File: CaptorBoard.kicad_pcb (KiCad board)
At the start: 2 copper layers, 90 x 50 mm, 56 parts, among them J2 Screw_Terminal_01x03, J3 Screw_Terminal_01x03, J5 Conn_01x04, J7 Conn_01x08, K1 G5LE-1-DC5, K2 G5LE-1-DC5, Q1 2N7002E, Q2 2N7002E, SW1 SW_PUSH, SW2 SW_PUSH, U1 ESP32-WROOM-32E-N4, U2 TC1264-3.3VDBTR, U3 MOC3041M-opto, U4 MOC3041M-opto, Y1 CM8V-T1A-32.768kHz-12.5pF-20P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

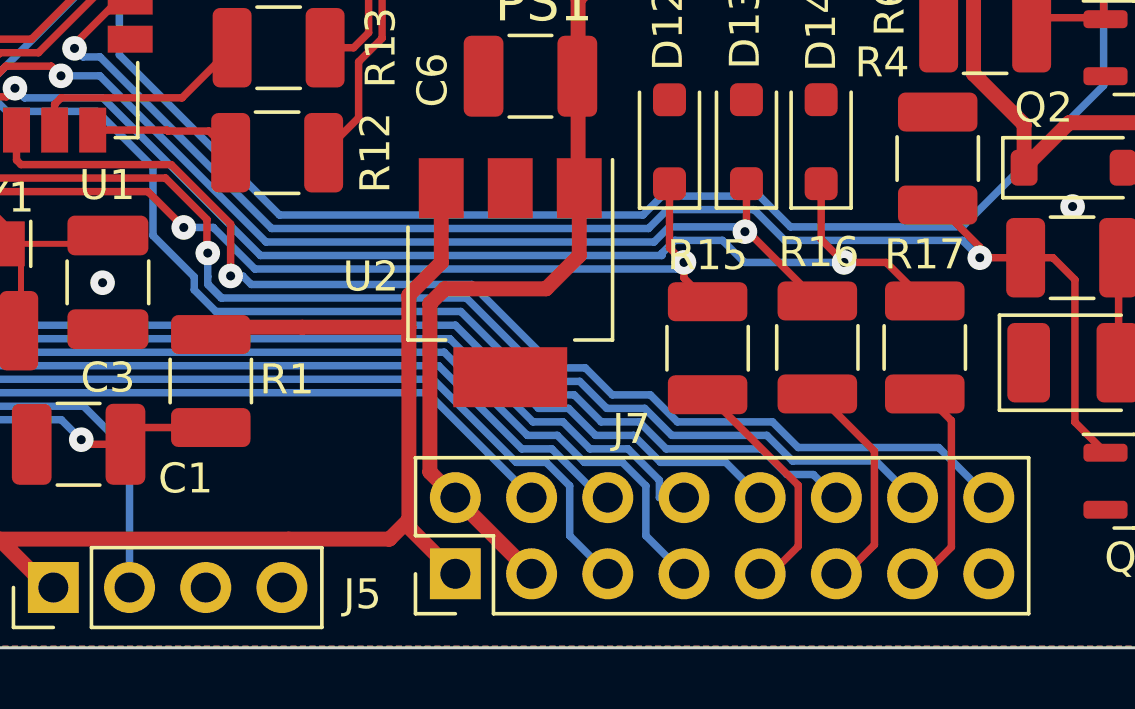
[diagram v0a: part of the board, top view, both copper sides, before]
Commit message: change route
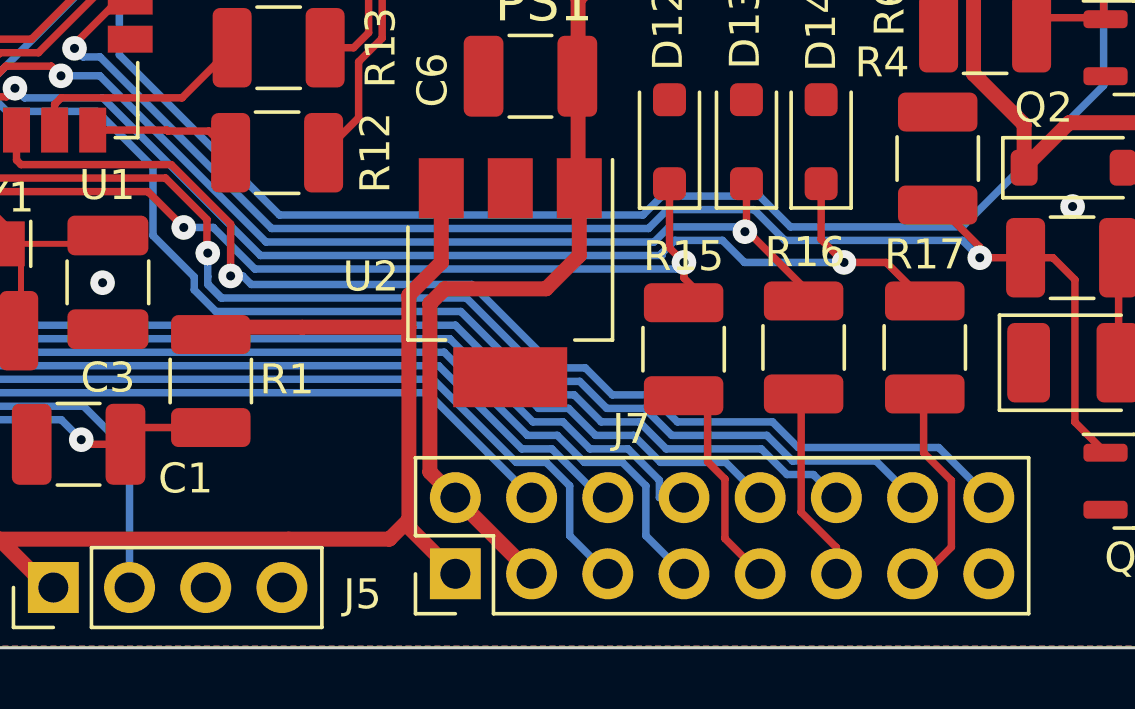
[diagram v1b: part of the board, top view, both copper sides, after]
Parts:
- moved R15 0.80 mm to (132.5, 90.0)
- moved R16 0.46 mm to (136.5, 90.0)
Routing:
- net Net-(J7-Pin_9): track 7.95 -> 6.69 mm
- net Net-(J7-Pin_11): track 7.49 -> 6.70 mm
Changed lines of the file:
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@@
   )
   (footprint "Resistor_SMD:R_1210_3225Metric_Pad1.30x2.65mm_HandSolder" (layer "F.Cu")
-    (at 133.2992 90.017 -90)
+    (at 132.5 90.05 -90)
     (descr "Resistor SMD 1210 (3225 Metric), square (rectangular) end terminal, IPC_7351 nominal with elongated pad for handsoldering. (Body size source: IPC-SM-782 page 72, https://www.pcb-3d.com/wordpress/wp-content/uploads/ipc-sm-782a_amendment_1_and_2.pdf), generated with kicad-footprint-generator")
     (tags "resistor handsolder")
@@
   )
   (footprint "Resistor_SMD:R_1210_3225Metric_Pad1.30x2.65mm_HandSolder" (layer "F.Cu")
-    (at 136.9568 89.9916 -90)
+    (at 136.5 89.9916 -90)
     (descr "Resistor SMD 1210 (3225 Metric), square (rectangular) end terminal, IPC_7351 nominal with elongated pad for handsoldering. (Body size source: IPC-SM-782 page 72, https://www.pcb-3d.com/wordpress/wp-content/uploads/ipc-sm-782a_amendment_1_and_2.pdf), generated with kicad-footprint-generator")
     (tags "resistor handsolder")
@@
     (pts (xy 185 50) (xy 185 100))
     (height -3.5)
-    (gr_text "50,0000 mm" (at 187.35 75 90) (layer "B.Fab")
+    (gr_text "50.0000 mm" (at 187.35 75 90) (layer "B.Fab")
       (effects (font (size 1 1) (thickness 0.15)))
     )
@@
     (pts (xy 95 50) (xy 185 50))
     (height -4.5)
-    (gr_text "90,0000 mm" (at 140 44.35) (layer "B.Fab")
+    (gr_text "90.0000 mm" (at 140 44.35) (layer "B.Fab")
       (effects (font (size 1 1) (thickness 0.15)))
     )
@@
   (segment (start 131.2418 94.604299) (end 131.2418 96.266) (width 0.25) (layer "B.Cu") (net 22))
   (segment (start 106.578569 90.15) (end 124.520388 90.15) (width 0.25) (layer "B.Cu") (net 22))
+  (segment (start 132.5118 87.1562) (end 132.0292 86.6736) (width 0.25) (layer "F.Cu") (net 23))
+  (segment (start 132.0292 86.6736) (end 132.0292 84.5342) (width 0.25) (layer "F.Cu") (net 23))
+  (segment (start 132.5118 87.6796) (end 133.2992 88.467) (width 0.25) (layer "F.Cu") (net 23))
   (segment (start 108.947957 84.346917) (end 108.743917 84.346917) (width 0.25) (layer "F.Cu") (net 23))
   (segment (start 108.743917 84.346917) (end 107.723 83.326) (width 0.25) (layer "F.Cu") (net 23))
   (segment (start 114.642462 84.7962) (end 109.39724 84.7962) (width 0.25) (layer "F.Cu") (net 23))
   (segment (start 115.837331 85.991069) (end 114.642462 84.7962) (width 0.25) (layer "F.Cu") (net 23))
-  (segment (start 132.5118 87.6796) (end 133.2992 88.467) (width 0.25) (layer "F.Cu") (net 23))
   (segment (start 107.723 83.326) (end 107.723 82.746) (width 0.25) (layer "F.Cu") (net 23))
-  (segment (start 132.0292 84.5342) (end 132.0292 86.6736) (width 0.25) (layer "F.Cu") (net 23))
   (segment (start 132.5118 87.1562) (end 132.5118 87.6796) (width 0.25) (layer "F.Cu") (net 23))
   (segment (start 109.39724 84.7962) (end 108.947957 84.346917) (width 0.25) (layer "F.Cu") (net 23))
-  (segment (start 132.0292 86.6736) (end 132.5118 87.1562) (width 0.25) (layer "F.Cu") (net 23))
   (via (at 115.837331 85.991069) (size 0.82) (drill 0.3) (layers "F.Cu" "B.Cu") (net 23))
   (via (at 132.5118 87.1562) (size 0.82) (drill 0.3) (layers "F.Cu" "B.Cu") (net 23))
-  (segment (start 116.822481 85.991069) (end 118.207412 87.376) (width 0.25) (layer "B.Cu") (net 23))
-  (segment (start 132.292 87.376) (end 132.5118 87.1562) (width 0.25) (layer "B.Cu") (net 23))
-  (segment (start 115.837331 85.991069) (end 116.822481 85.991069) (width 0.25) (layer "B.Cu") (net 23))
-  (segment (start 118.207412 87.376) (end 132.292 87.376) (width 0.25) (layer "B.Cu") (net 23))
+  (segment (start 132.292 87.376) (end 118.207412 87.376) (width 0.25) (layer "B.Cu") (net 23))
+  (segment (start 118.207412 87.376) (end 116.822481 85.991069) (width 0.25) (layer "B.Cu") (net 23))
+  (segment (start 132.5118 87.1562) (end 132.292 87.376) (width 0.25) (layer "B.Cu") (net 23))
+  (segment (start 116.822481 85.991069) (end 115.837331 85.991069) (width 0.25) (layer "B.Cu") (net 23))
   (segment (start 99.469161 80.9498) (end 100.133261 80.2857) (width 0.25) (layer "F.Cu") (net 24))
   (segment (start 112.4276 70.821843) (end 111.533 69.927243) (width 0.25) (layer "F.Cu") (net 24))
@@
   (segment (start 110.758 64.171) (end 110.263 64.666) (width 0.25) (layer "F.Cu") (net 35))
   (segment (start 109.906153 80.6157) (end 109.336153 81.1857) (width 0.25) (layer "F.Cu") (net 36))
-  (segment (start 134.646953 86.131753) (end 134.543447 86.131753) (width 0.25) (layer "F.Cu") (net 36))
   (segment (start 100.103 81.746) (end 100.103 82.746) (width 0.25) (layer "F.Cu") (net 36))
   (segment (start 100.6633 81.1857) (end 100.103 81.746) (width 0.25) (layer "F.Cu") (net 36))
   (segment (start 109.336153 81.1857) (end 100.6633 81.1857) (width 0.25) (layer "F.Cu") (net 36))
   (segment (start 134.5946 86.0806) (end 134.543447 86.131753) (width 0.25) (layer "F.Cu") (net 36))
-  (segment (start 136.9568 88.4416) (end 134.646953 86.131753) (width 0.25) (layer "F.Cu") (net 36))
   (segment (start 134.5946 84.5312) (end 134.5946 86.0806) (width 0.25) (layer "F.Cu") (net 36))
   (segment (start 111.746071 80.9365) (end 111.425271 80.6157) (width 0.25) (layer "F.Cu") (net 36))
+  (segment (start 134.646953 86.131753) (end 134.543447 86.131753) (width 0.25) (layer "F.Cu") (net 36))
   (segment (start 111.425271 80.6157) (end 109.906153 80.6157) (width 0.25) (layer "F.Cu") (net 36))
+  (segment (start 136.9568 88.4416) (end 134.646953 86.131753) (width 0.25) (layer "F.Cu") (net 36))
   (via (at 111.746071 80.9365) (size 0.82) (drill 0.3) (layers "F.Cu" "B.Cu") (net 36))
   (via (at 134.543447 86.131753) (size 0.82) (drill 0.3) (layers "F.Cu" "B.Cu") (net 36))
@@
   (segment (start 132.290481 92.471) (end 135.461293 92.471) (width 0.25) (layer "B.Cu") (net 65))
   (segment (start 135.461293 92.471) (end 136.317093 93.3268) (width 0.25) (layer "B.Cu") (net 65))
-  (segment (start 135.405447 97.536) (end 135.0518 97.536) (width 0.25) (layer "F.Cu") (net 66))
-  (segment (start 136.3202 94.588) (end 136.3202 96.621247) (width 0.25) (layer "F.Cu") (net 66))
-  (segment (start 133.2992 91.567) (end 136.3202 94.588) (width 0.25) (layer "F.Cu") (net 66))
-  (segment (start 136.3202 96.621247) (end 135.405447 97.536) (width 0.25) (layer "F.Cu") (net 66))
-  (segment (start 137.894647 97.536) (end 137.5918 97.536) (width 0.25) (layer "F.Cu") (net 67))
-  (segment (start 138.8602 93.445) (end 138.8602 96.570447) (width 0.25) (layer "F.Cu") (net 67))
-  (segment (start 138.8602 96.570447) (end 137.894647 97.536) (width 0.25) (layer "F.Cu") (net 67))
-  (segment (start 136.9568 91.5416) (end 138.8602 93.445) (width 0.25) (layer "F.Cu") (net 67))
-  (segment (start 140.536247 97.536) (end 140.1318 97.536) (width 0.25) (layer "F.Cu") (net 68))
-  (segment (start 140.5382 91.5416) (end 141.4256 92.429) (width 0.25) (layer "F.Cu") (net 68))
+  (segment (start 133.2992 93.7992) (end 133.8768 94.3768) (width 0.25) (layer "F.Cu") (net 66))
+  (segment (start 133.8768 96.361) (end 135.0518 97.536) (width 0.25) (layer "F.Cu") (net 66))
+  (segment (start 133.8768 94.3768) (end 133.8768 96.361) (width 0.25) (layer "F.Cu") (net 66))
+  (segment (start 133.2992 91.567) (end 133.2992 93.7992) (width 0.25) (layer "F.Cu") (net 66))
+  (segment (start 137.5918 96.657701) (end 137.5918 97.536) (width 0.25) (layer "F.Cu") (net 67))
+  (segment (start 136.4168 95.482701) (end 137.5918 96.657701) (width 0.25) (layer "F.Cu") (net 67))
+  (segment (start 136.4168 92.0816) (end 136.4168 95.482701) (width 0.25) (layer "F.Cu") (net 67))
+  (segment (start 136.9568 91.5416) (end 136.4168 92.0816) (width 0.25) (layer "F.Cu") (net 67))
+  (segment (start 141.4256 94.4256) (end 141.4256 96.646647) (width 0.25) (layer "F.Cu") (net 68))
+  (segment (start 140.5 93.5) (end 141.4256 94.4256) (width 0.25) (layer "F.Cu") (net 68))
   (segment (start 141.4256 96.646647) (end 140.536247 97.536) (width 0.25) (layer "F.Cu") (net 68))
-  (segment (start 141.4256 92.429) (end 141.4256 96.646647) (width 0.25) (layer "F.Cu") (net 68))
+  (segment (start 140.5 91.5798) (end 140.5 93.5) (width 0.25) (layer "F.Cu") (net 68))
+  (segment (start 140.5382 91.5416) (end 140.5 91.5798) (width 0.25) (layer "F.Cu") (net 68))
+  (segment (start 140.536247 97.536) (end 140.1318 97.536) (width 0.25) (layer "F.Cu") (net 68))
   (zone (net 9) (net_name "GND") (layers "F&B.Cu") (hatch edge 0.508)
     (priority 3)
